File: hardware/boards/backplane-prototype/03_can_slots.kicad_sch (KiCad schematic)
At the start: 15 parts, among them J1 SLOT_1, J2 XY308-2.54-3P / EXTERNAL CAN, J3 SLOT_2, J4 SLOT_3, J6 SLOT_4, J7 SLOT_5, J8 SLOT_6, U5 TCAN3413DR

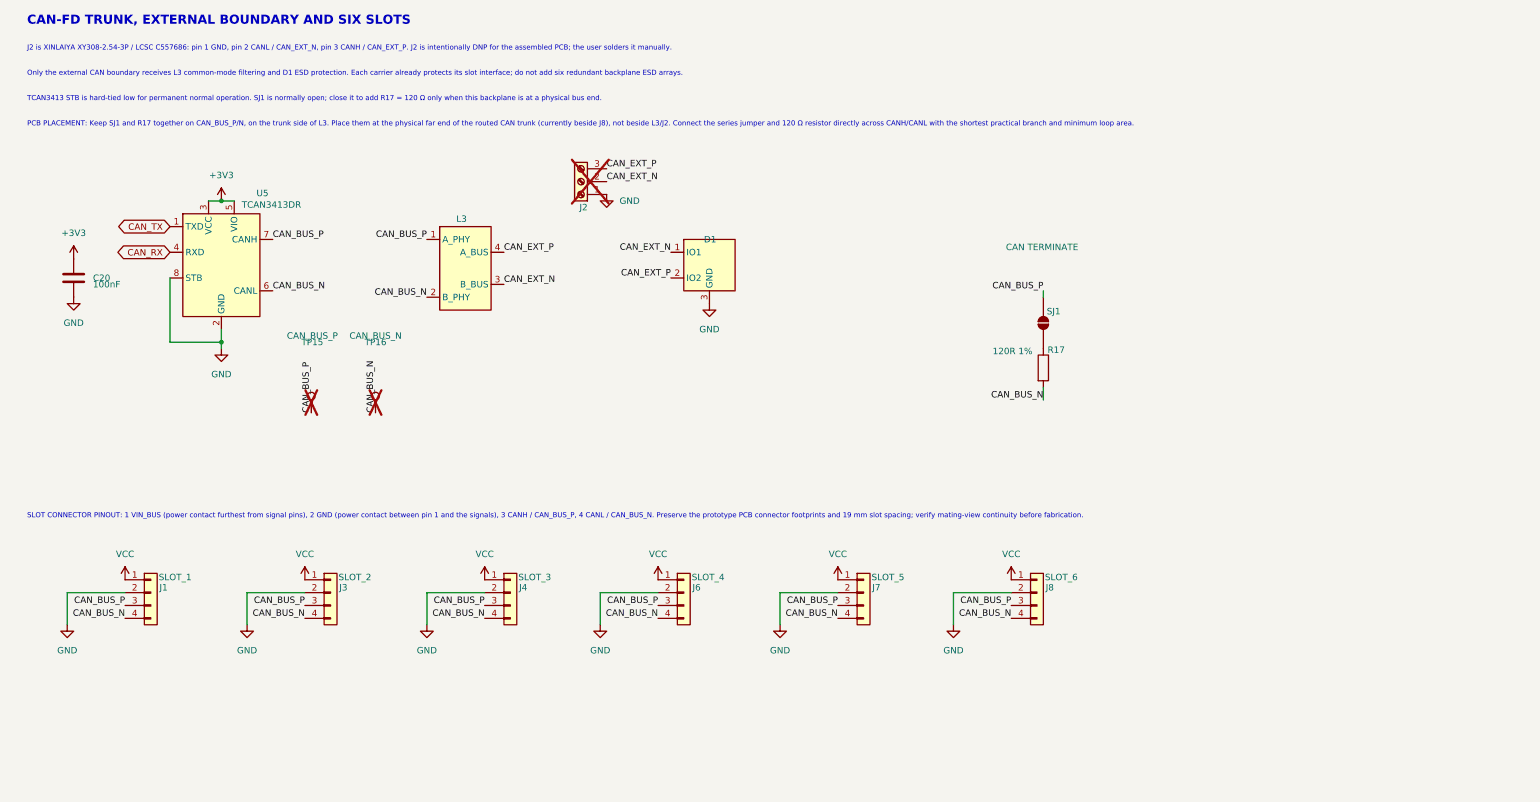
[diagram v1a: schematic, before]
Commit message: checkpoint: save schematic updates
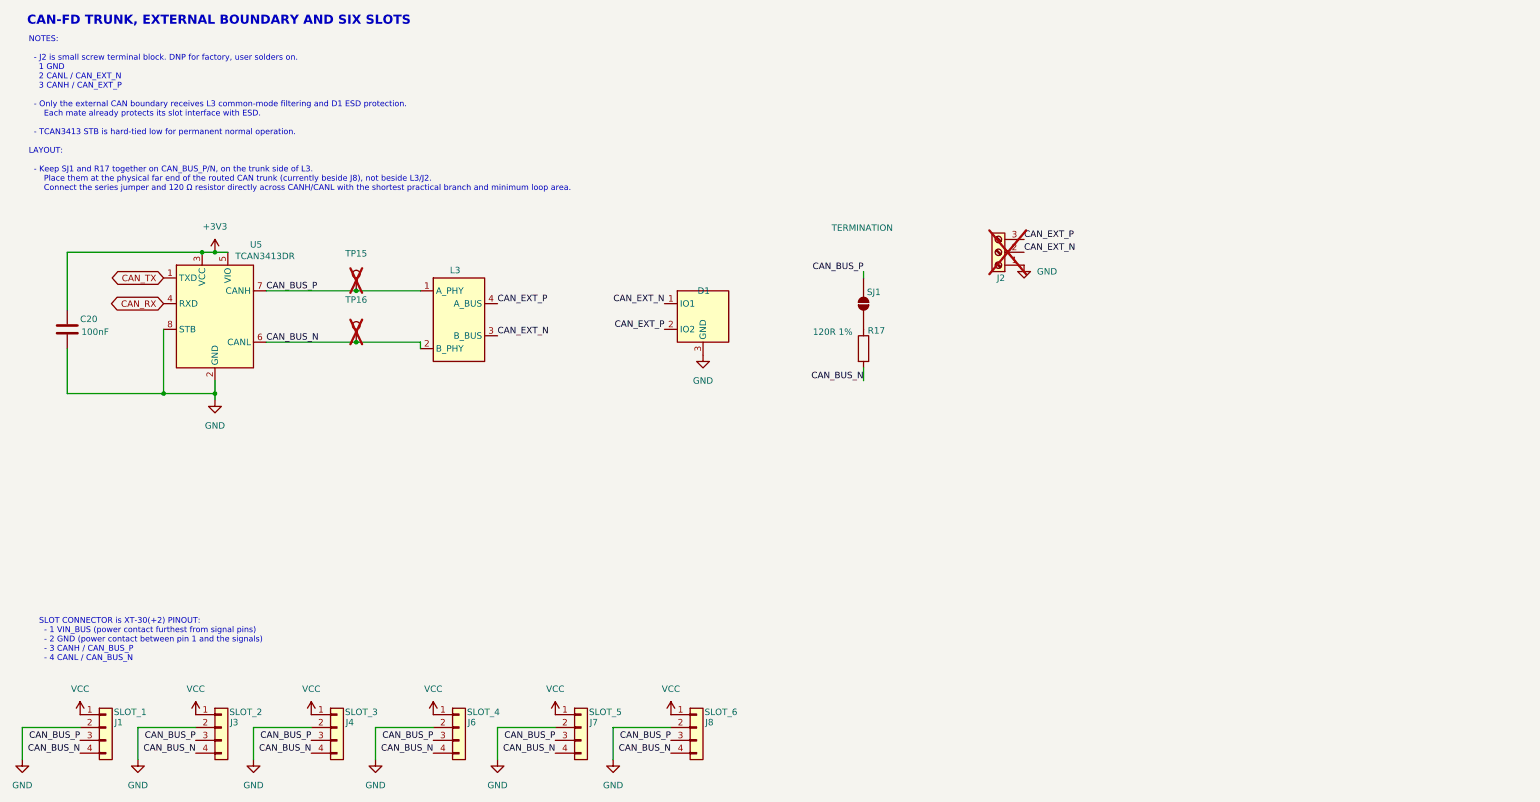
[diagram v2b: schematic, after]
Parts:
- SJ1: value CAN TERMINATE -> TERMINATION
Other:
- note added: "NOTES: - J2 is small screw terminal block. DNP for factory, user solders on. 1 GND 2 CANL / CAN_EXT_N 3 CANH / CAN_EXT_P - Only the external CAN boundary receives L3 common-mode filtering and D1 ESD protection. Each mate already protects its slot interface with ESD. - TCAN3413 STB is hard-tied low for permanent normal operation. LAYOUT: - Keep SJ1 and R17 together on CAN_BUS_P/N, on the trunk sid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"
- note added: "SLOT CONNECTOR is XT-30(+2) PINOUT: - 1 VIN_BUS (power contact furthest from signal pins) - 2 GND (power contact between pin 1 and the signals) - 3 CANH / CAN_BUS_P - 4 CANL / CAN_BUS_N"
- note removed: "J2 is XINLAIYA XY308-2.54-3P / LCSC C557686: pin 1 GND, pin 2 CANL / CAN_EXT_N, pin 3 CANH / CAN_EXT_P. J2 is intentionally DNP for the assembled PCB; the user solders it manually."
- note removed: "Only the external CAN boundary receives L3 common-mode filtering and D1 ESD protection. Each carrier already protects its slot interface; do not add six redundant backplane ESD arrays."
- note removed: "PCB PLACEMENT: Keep SJ1 and R17 together on CAN_BUS_P/N, on the trunk side of L3. Place them at the physical far end of the routed CAN trunk (currently beside J8), not beside L3/J2. Connect the series jumper and 120 Ω resistor directly across CANH/CANL with the shortest practical branch and minimum loop area."
- note removed: "SLOT CONNECTOR PINOUT: 1 VIN_BUS (power contact furthest from signal pins), 2 GND (power contact between pin 1 and the signals), 3 CANH / CAN_BUS_P, 4 CANL / CAN_BUS_N. Preserve the prototype PCB connector footprints and 19 mm slot spacing; verify mating-view continuity before fabrication."
- note removed: "TCAN3413 STB is hard-tied low for permanent normal operation. SJ1 is normally open; close it to add R17 = 120 Ω only when this backplane is at a physical bus end."
- moved on the sheet: C20, D1, J1, J2, J3, J4, J6, J7, J8, L3, R17, SJ1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
